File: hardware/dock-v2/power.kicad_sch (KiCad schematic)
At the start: 27 parts, among them J101 TYPE-C-31-M-12, U101 TPD4E1U06DBVR, U102 CH224A, U103 TPS54331DR, U104 AMS1117-3.3

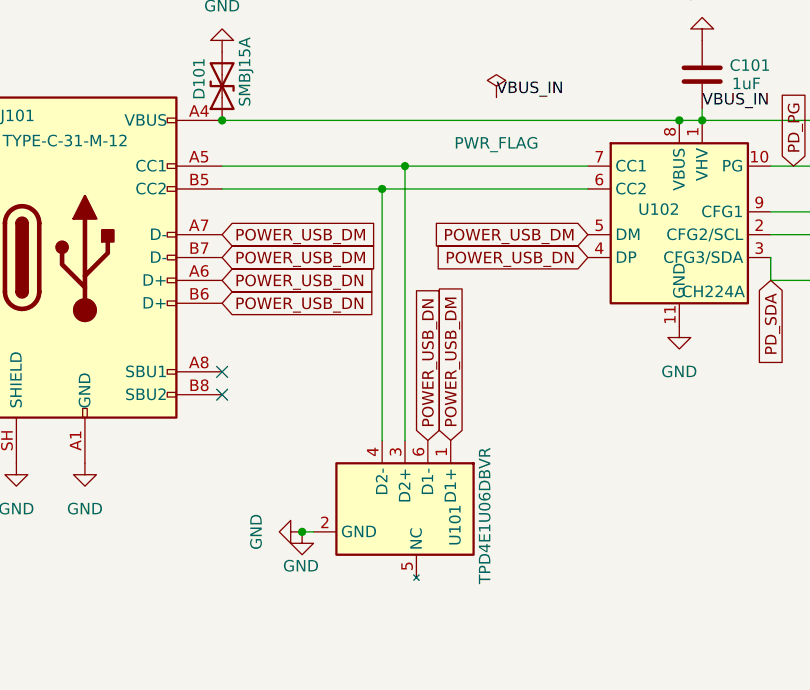
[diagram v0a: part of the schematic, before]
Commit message: Dock v2: PCB placement in progress (user's work, snapshot)
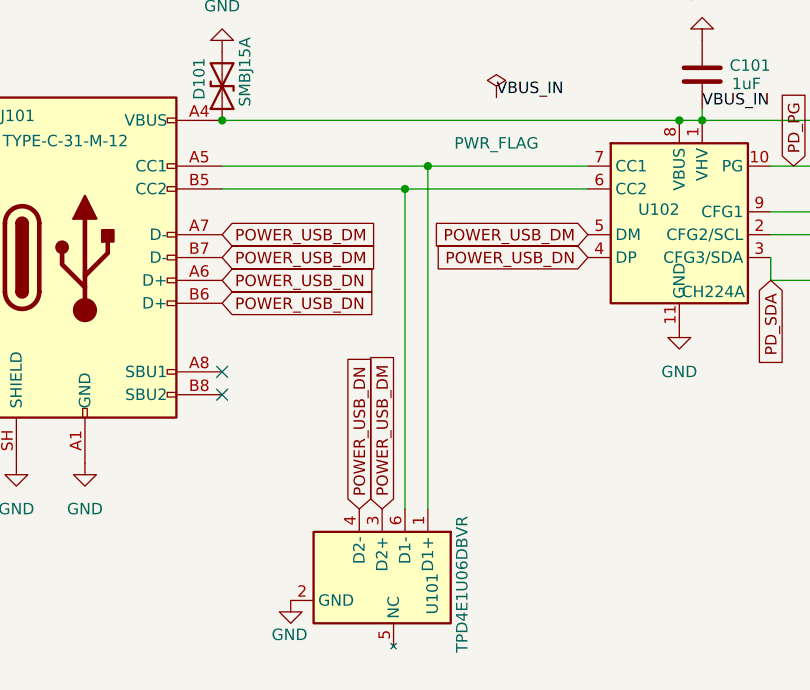
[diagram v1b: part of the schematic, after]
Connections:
- net POWER_USB_DM: now also U101.3 (D2+); no longer U101.1 (D1+)
- net POWER_USB_DN: now also U101.4 (D2-); no longer U101.6 (D1-)
- net at J101.B5 (CC2), U102.6 (CC2): now also U101.6 (D1-); no longer U101.4 (D2-)
- net at J101.A5 (CC1), U102.7 (CC1): now also U101.1 (D1+); no longer U101.3 (D2+)
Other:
- moved on the sheet: U101
